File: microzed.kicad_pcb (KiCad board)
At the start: 10 copper layers, 60 x 100 mm, 336 parts, among them IC1 XC7Z020-1CLG484C, IC2 RTL8211E-VL-CG, J1 640456-3, J2 10104111-0001LF, J3 L829-1J1T-43, J4 Micro_SD_Card_Det_Hirose_DM3AT, J5 10104111-0001LF, J6 BSH-090-01-X-D-A, J7 BSH-090-01-X-D-A, Q1 MMBT3904, Q2 MMBT3904, Q3 BSS138, SW1 SW_Push, U1 TLV62130RGTR, U10 MT41K256M16TW, U11 MT25QL128ABA8E12-1SIT, U12 USB3320C-EZK, U13 ASDMB-24.000MHZ-LC-T, U14 ASDMB-25.000MHZ-LC-T, U15 TXS02612RTWR, U16 CP2104-F03-GM, U2 TLV62130RGTR, U3 TLV62130RGTR, U4 TLV62130RGTR, U5 TLV62130RGTR, U6 ASDMB-33.333MHZ-LC-T, U7 TPS51206DSQR, U8 REF3012, U9 MT41K256M16TW

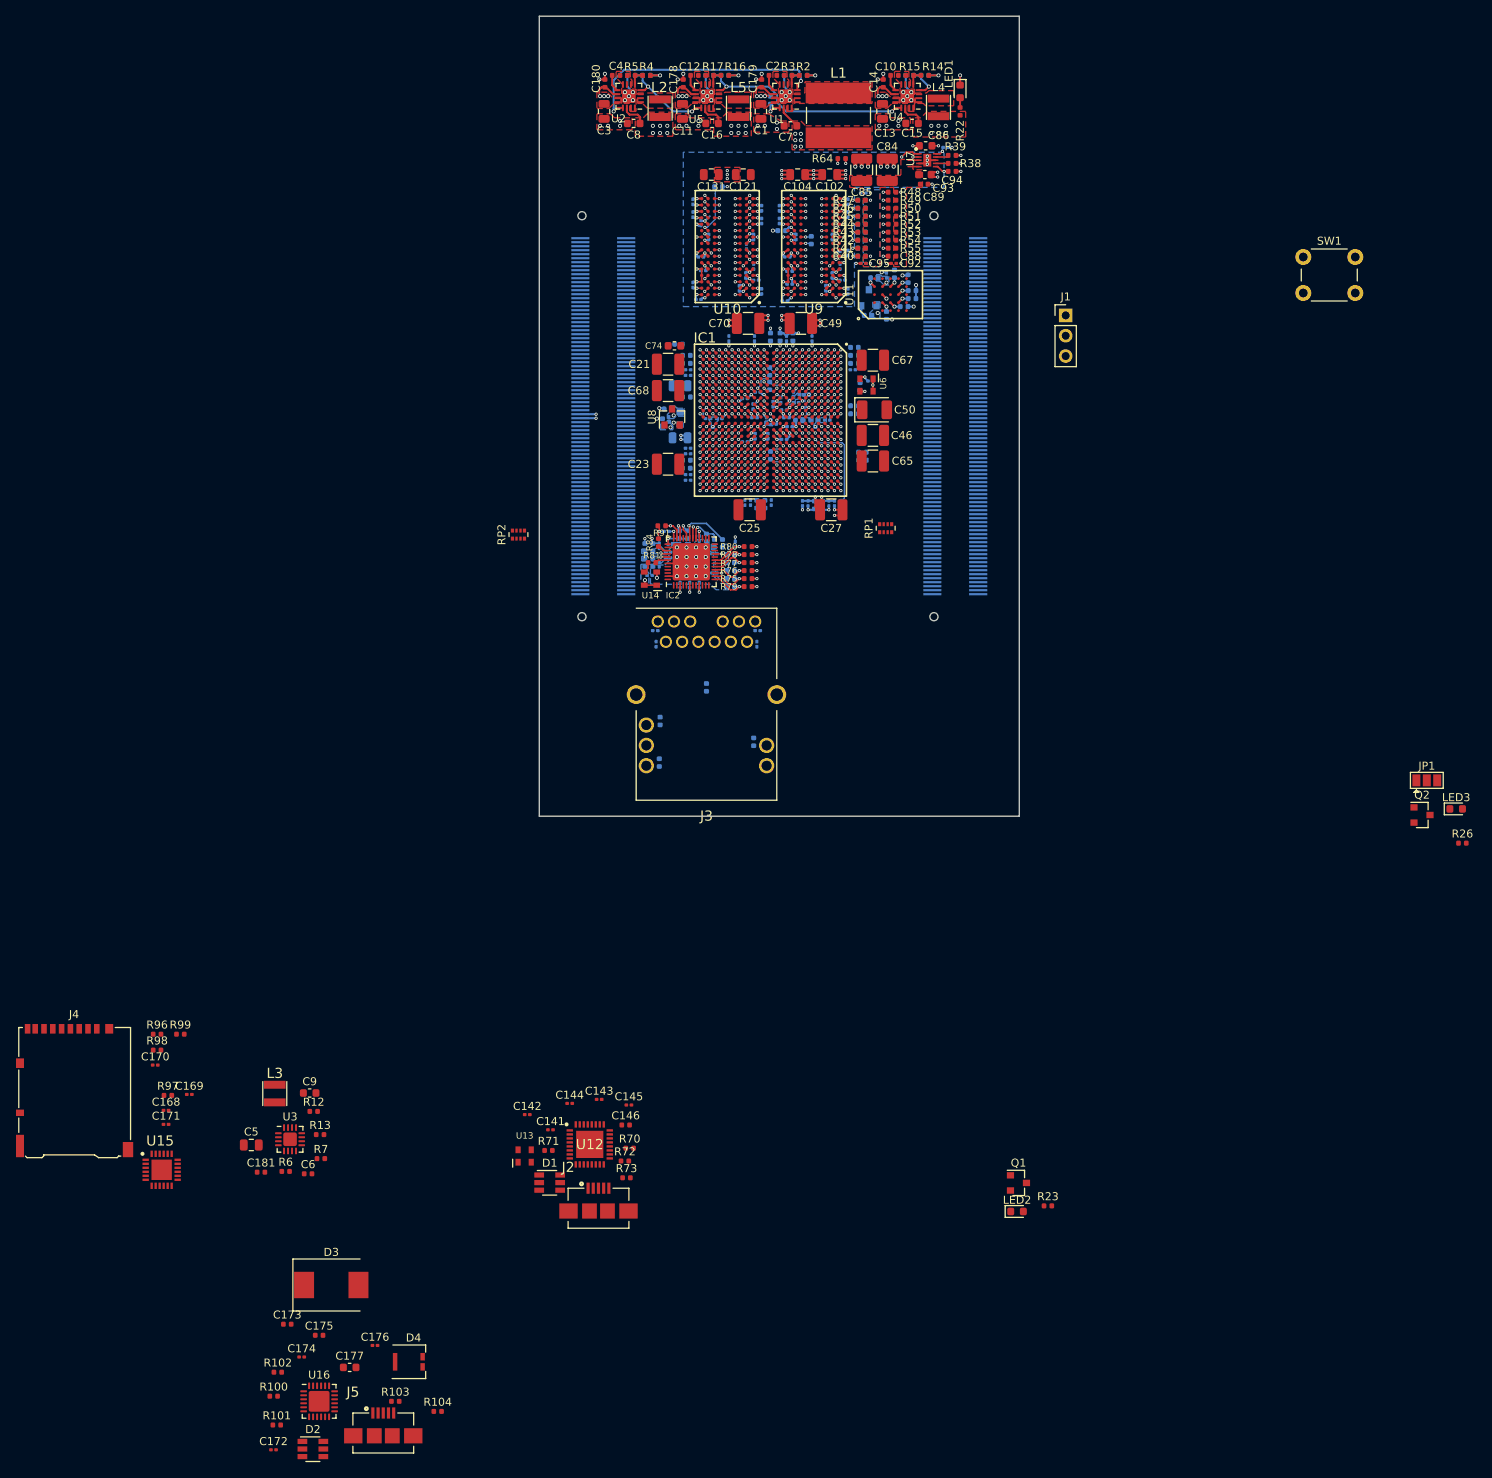
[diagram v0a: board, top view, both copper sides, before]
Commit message: elements located nearly done
Signed-off-by: Yi Qingliang <niqingliang2003@gmail.com>
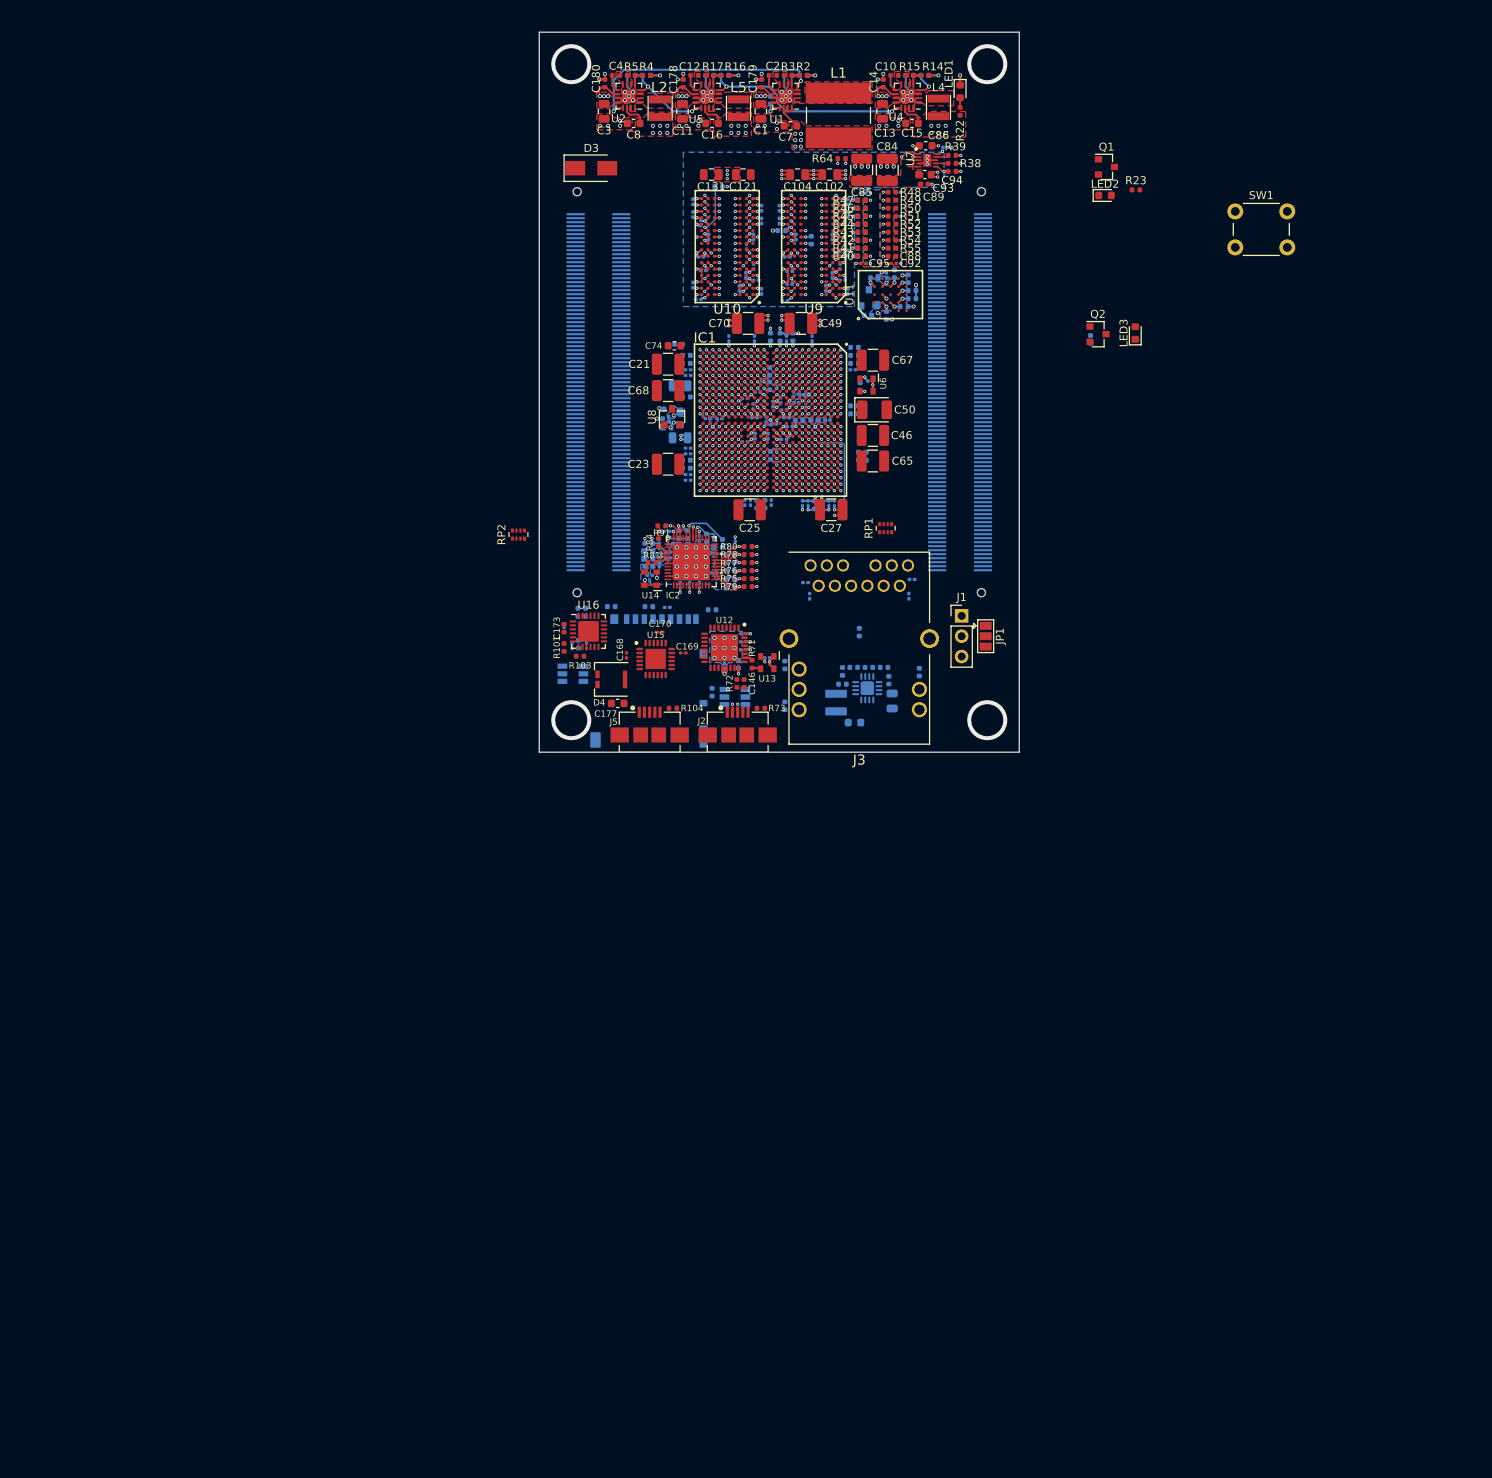
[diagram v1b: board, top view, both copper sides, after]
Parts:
- C141, C142, C143, C144, C145, C171, C172, C174, C175, C176, C181, C5, C6, C9, D1, D2, J4, L3, R100, R102, R12, R13, R26, R6, R7, R70, R96, R97, R98, R99, U3: moved to B.Cu
- D3: footprint Diode_SMD:D_SMC -> Diode_SMD:D_SMA
- moved D3 143.3 mm to (-23.5, 19.0)
- moved LED2 127.5 mm to (40.7, 22.4)
- moved Q1 127.5 mm to (40.9, 18.8)
- moved R23 127.5 mm to (44.6, 21.7)
- moved C172 107.8 mm to (-24.1, 78.7), turned to 90 degrees
- moved R100 105.8 mm to (-24.7, 74.0)
- moved R101 103.6 mm to (-26.9, 78.9), turned to 270 degrees
- moved D2 102.2 mm to (-25.8, 82.2)
- moved U16 102.0 mm to (-23.9, 76.9)
- moved R102 101.8 mm to (-24.7, 75.0)
- moved C181 99.7 mm to (13.7, 83.0), turned to 270 degrees
- moved C5 97.4 mm to (14.1, 85.6), turned to 270 degrees
- moved C174 96.6 mm to (-26.9, 76.7), turned to 90 degrees
- moved R103 96.0 mm to (-24.9, 80.0), turned to 180 degrees
- moved C6 95.9 mm to (13.1, 81.4)
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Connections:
- Q3 pad 2: CARRIER_SRST# -> Net-(Q3-Pad2)
- Q3 pad 3: Net-(Q3-Pad3) -> CARRIER_SRST#
- R106 pad 2: Net-(Q3-Pad3) -> CARRIER_SRST#
- U11 pad A4: Net-(Q3-Pad3) -> CARRIER_SRST#
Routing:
- net PWR_B501: track 22.9 -> 29.4 mm, vias 21 -> 25
- net V3V3: track 32.4 -> 34.8 mm, vias 26 -> 27
- net Net-(Q3-Pad3): track 2.30 -> 0.00 mm, vias 1 -> 0
- net CARRIER_SRST#: track 1.92 -> 4.21 mm, vias 1 -> 2
- net BANK13_LVDS_6_N: track 2.53 -> 0.57 mm, vias 2 -> 1
- net Net-(R70-Pad1): track 0.00 -> 1.47 mm, vias 0 -> 1
- net Net-(R71-Pad1): track 0.00 -> 1.08 mm
- net Net-(R71-Pad2): track 0.00 -> 0.98 mm
- net GND: track 148.5 -> 148.0 mm, vias 203 -> 211
- net Net-(C175-Pad1): vias 0 -> 1
- net (no net): vias 0 -> 6
- added copper zone on In8.Cu.VCC, net GND
- removed copper zone on In8.Cu.VCC, net VIN
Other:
- board size 60 x 100 mm -> 60 x 90 mm
